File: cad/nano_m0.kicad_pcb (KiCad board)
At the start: 2 copper layers, 34.3 x 45.1 mm, 29 parts, among them J1 Conn_01x10, J2 Conn_01x10, J3 USB_B_Micro, J4 SWD, SW1 SW_SPST, SW2 SW_SPST, U1 AP2112K-3.3TRG1, U2 STM32F0706P6, Y1 16MHz

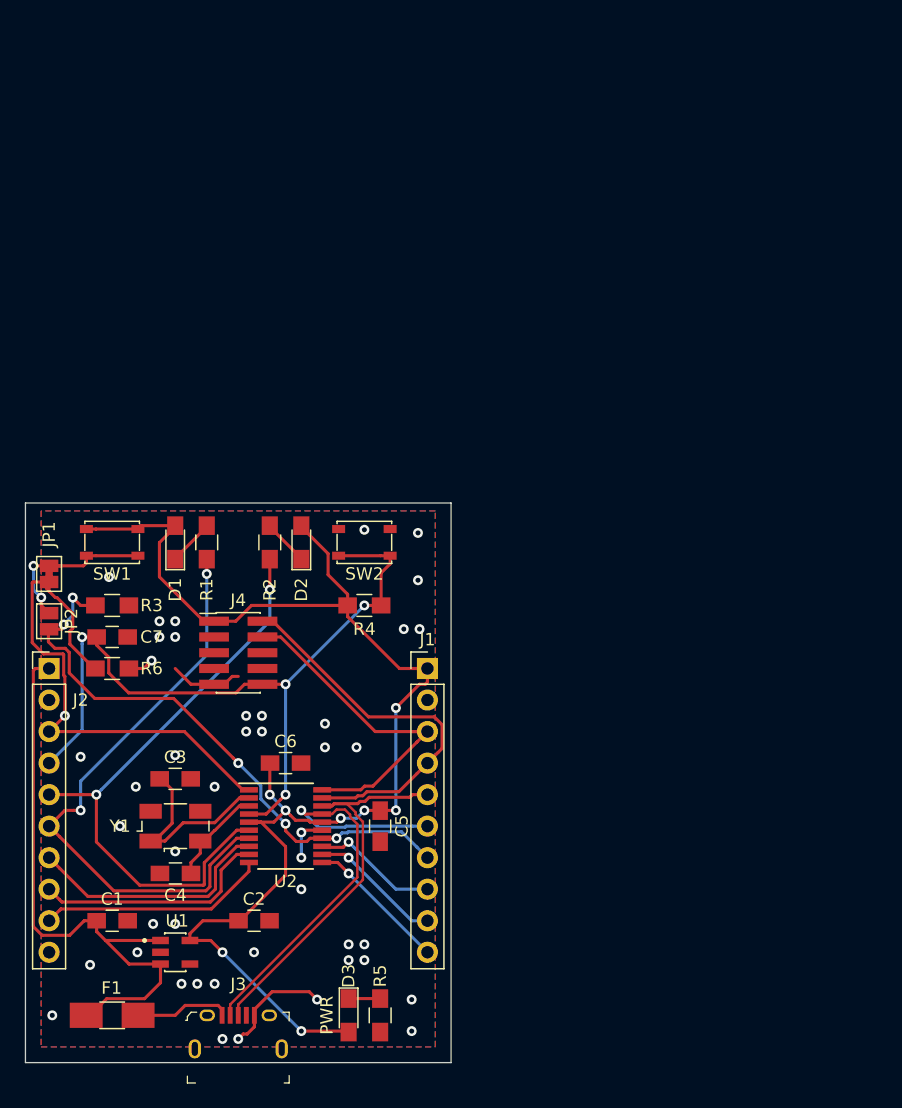
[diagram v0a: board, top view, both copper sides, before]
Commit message: board v2
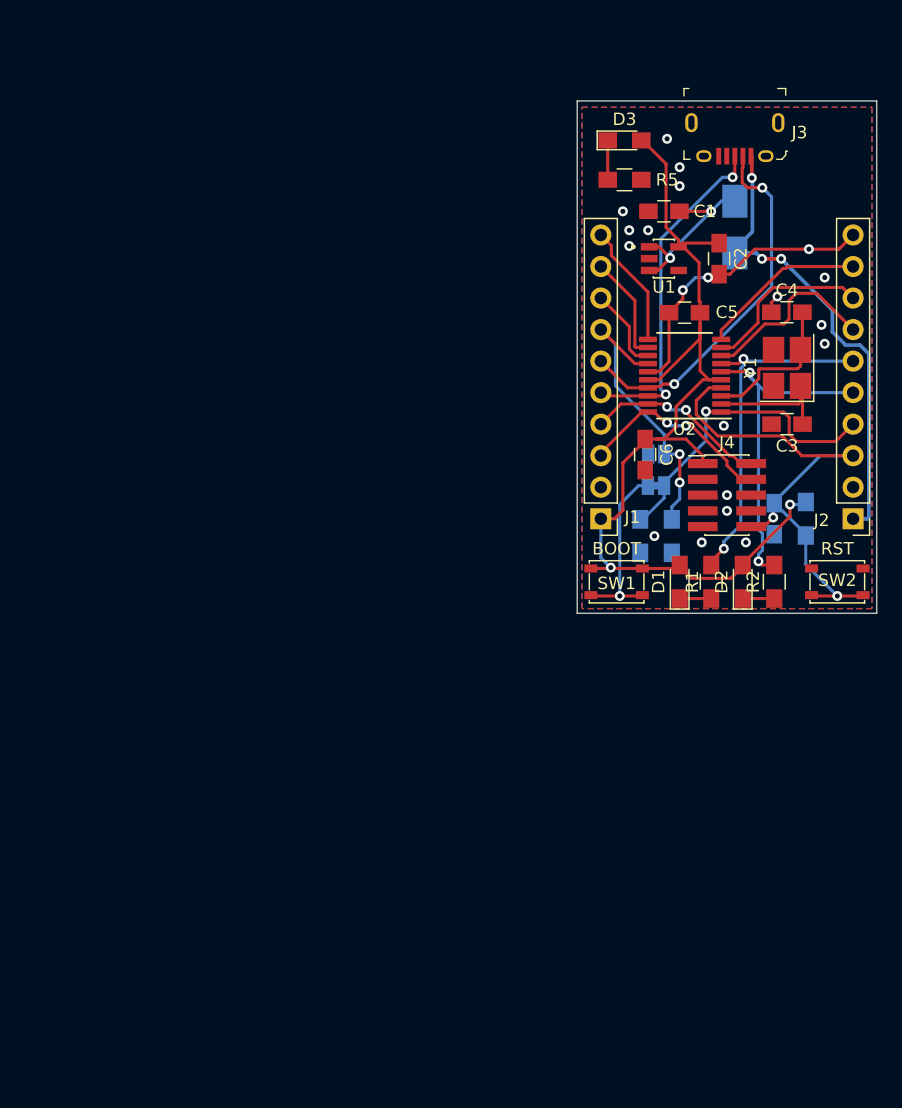
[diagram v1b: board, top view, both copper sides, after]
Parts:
- removed the REF*** at (120.0, 108.6)
- added REF***: OSHW-Symbol_6.7x6mm_SilkScreen, Symbols:OSHW-Symbol_6.7x6mm_SilkScreen, B.Cu at (143.3, 72.6)
- C3, C4: value 15pF -> 22pF
- C7, F1, JP1, JP2, R3, R4, R6: moved to B.Cu
- U1: value AP2112K-3.3TRG1 -> (none)
- Y1: value 16MHz -> Crystal; footprint Crystals:Crystal_SMD_Abracon_ABM3B-4pin_5.0x3.2mm -> Crystals:Crystal_SMD_SeikoEpson_TSX3225-4pin_3.2x2.5mm_HandSoldering
- moved F1 80.9 mm to (151.8, 78.7), turned to 270 degrees
- moved J3 79.9 mm to (151.8, 73.0), turned to 180 degrees
- moved D3 73.9 mm to (142.9, 71.8), turned to 0 degrees
- moved C1 72.4 mm to (146.1, 77.5), turned to 180 degrees
- moved R5 70.1 mm to (142.9, 74.9), turned to 0 degrees
- moved U1 68.4 mm to (146.1, 81.3)
- moved C4 66.9 mm to (156.0, 85.6)
- moved J2 65.9 mm to (161.3, 102.2), turned to 180 degrees
- moved C2 65.2 mm to (150.5, 81.3), turned to 270 degrees
- moved Y1 61.6 mm to (156.0, 90.1), turned to 90 degrees
- moved C3 57.0 mm to (156.0, 94.6), turned to 180 degrees
- moved C7 54.2 mm to (154.9, 102.2), turned to 270 degrees
- moved JP2 50.7 mm to (145.4, 97.0), turned to 0 degrees
- moved JP1 49.4 mm to (145.4, 99.6), turned to 0 degrees
- moved U2 48.5 mm to (147.7, 90.7), turned to 180 degrees
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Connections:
- C1 pad 1: +5V -> Net-(C1-Pad1)
- F1 pad 1: +5V -> Net-(C1-Pad1)
- F1 pad 2: VBUS -> +5V
- J2 pad 3: /BOOT -> /NRST
- J2 pad 4: /NRST -> /BOOT
- J3 pad 1: VBUS -> +5V
- U1 pad 1: +5V -> Net-(C1-Pad1)
- U1 pad 3: +5V -> Net-(C1-Pad1)
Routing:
- net +3V3: track 108.4 -> 81.0 mm, vias 8 -> 2
- net /PB1: track 47.4 -> 24.1 mm, vias 5 -> 2
- net /PA0: track 49.2 -> 28.4 mm
- net /PA1: track 48.5 -> 28.5 mm
- net /NRST: track 62.2 -> 42.6 mm, vias 4 -> 2
- net /BOOT: track 43.1 -> 25.2 mm
- net /PA13: track 31.1 -> 14.9 mm, vias 0 -> 2
- net Net-(C1-Pad1): track 0.00 -> 14.1 mm, vias 0 -> 2
- net /PA14: track 28.1 -> 16.5 mm, vias 0 -> 2
- net +5V: track 47.9 -> 38.1 mm, vias 0 -> 3
- net VBUS: track 7.71 -> 0.00 mm
- net /USB_N: track 35.8 -> 30.3 mm, vias 1 -> 2
- net /PA2: track 20.1 -> 14.8 mm
- net /PA3: track 19.1 -> 13.9 mm
- net /PA4: track 18.5 -> 13.5 mm
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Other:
- board size 34.3 x 45.1 mm -> 24.1 x 41.3 mm
- net class POWER added: clearance 0.25, trace_width 0.3, via_dia 0.8, via_drill 0.4
- board text added: "3.3V"
- board text added: "5V"
- board text added: "BOOT"
- board text added: "GND"
- board text added: "NANO-M0 @ZKLAPOW"
- board text added: "PA0"
- board text added: "PA1"
- board text added: "PA13"
- board text added: "PA14"
- board text added: "PA2"
- board text added: "PA3"
- board text added: "PA4"
- board text added: "PA5"
- board text added: "PA6"
- board text added: "PA7"
- board text added: "PB1"
- board text added: "RST"
- board text added: "USB_N"
- board text added: "USB_P"
- board text added: "V2"
- board text removed: "@zklapow"
- board text removed: "NANO-M0"
- board text removed: "V1"

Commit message: final v3 board
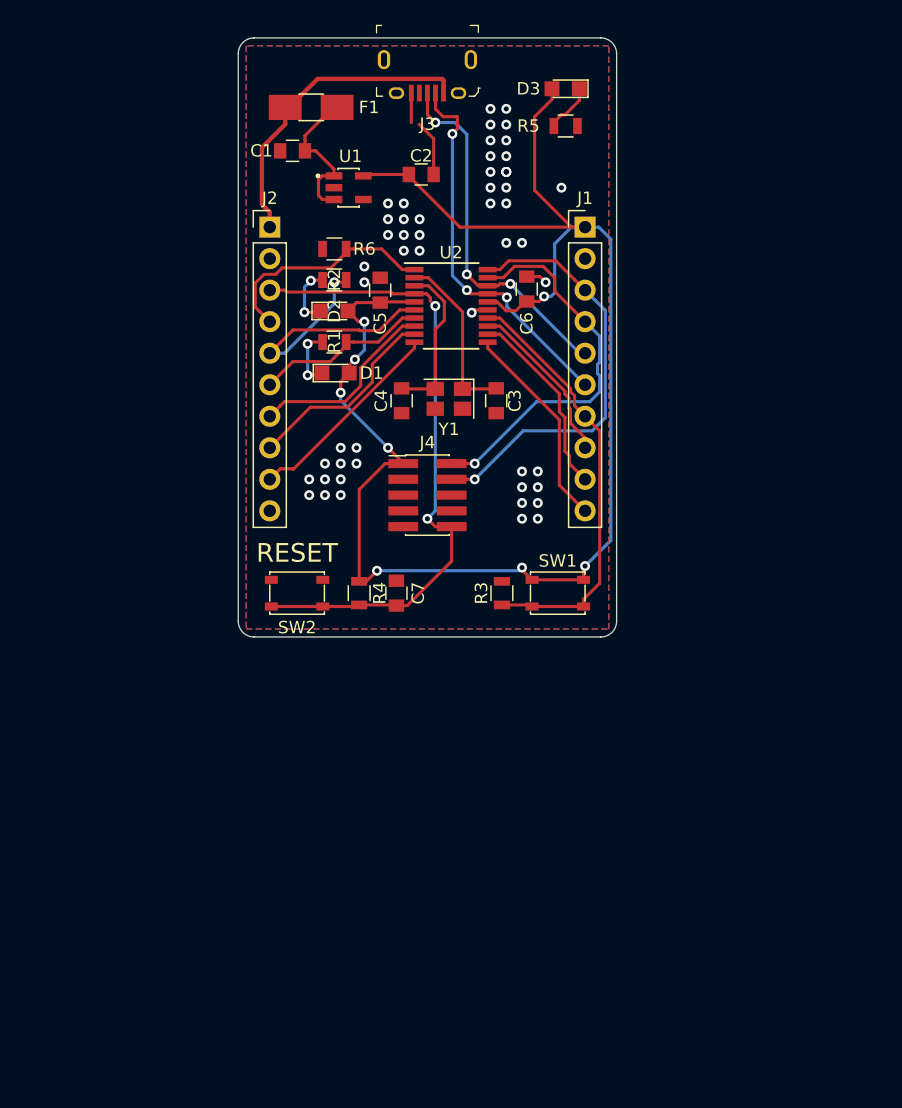
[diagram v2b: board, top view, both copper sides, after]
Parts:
- removed JP1: Jumper_NC_Small, Jumper:SolderJumper-2_P1.3mm_Bridged_Pad1.0x1.5mm
- removed JP2: Jumper_NO_Small, Jumper:SolderJumper-2_P1.3mm_Open_Pad1.0x1.5mm
- removed REF***: OSHW-Symbol_6.7x6mm_SilkScreen, Symbols:OSHW-Symbol_6.7x6mm_SilkScreen
- C1, C2, C3, C4, C5, C6: footprint Capacitors_SMD:C_0805_HandSoldering -> Capacitors_SMD:C_0805
- C7: footprint Capacitors_SMD:C_0805_HandSoldering -> Capacitors_SMD:C_0805; moved to F.Cu
- D1, D2, D3: footprint LEDs:LED_0805_HandSoldering -> LEDs:LED_0805
- F1: moved to F.Cu
- R1, R2, R5: value 80ohm -> 100; footprint Resistors_SMD:R_0805_HandSoldering -> Resistors_SMD:R_0805
- R3, R4, R6: footprint Resistors_SMD:R_0805_HandSoldering -> Resistors_SMD:R_0805; moved to F.Cu
- U1: value (none) -> AP2112K-3.3TRG1
- Y1: footprint Crystals:Crystal_SMD_SeikoEpson_TSX3225-4pin_3.2x2.5mm_HandSoldering -> Crystals:Crystal_SMD_SeikoEpson_TSX3225-4pin_3.2x2.5mm
- moved J2 52.5 mm to (114.3, 78.7), turned to 0 degrees
- moved SW2 43.5 mm to (116.5, 108.2)
- moved R2 43.0 mm to (119.5, 83.0), turned to 0 degrees
- moved D2 39.5 mm to (119.5, 85.5), turned to 0 degrees
- moved R4 36.5 mm to (121.5, 108.2)
- moved R1 36.0 mm to (119.5, 88.0), turned to 0 degrees
- moved F1 35.5 mm to (117.6, 69.1), turned to 180 degrees
- moved R6 33.8 mm to (119.5, 80.5), turned to 180 degrees
- moved D1 32.4 mm to (119.6, 90.5), turned to 0 degrees
- moved C4 31.8 mm to (124.9, 92.7), turned to 270 degrees
- moved C7 31.0 mm to (124.5, 108.2), turned to 90 degrees
- moved C1 30.3 mm to (116.1, 72.6)
- moved Y1 27.4 mm to (128.7, 92.6), turned to 180 degrees
- moved U1 26.0 mm to (120.7, 75.6)
- moved J3 25.3 mm to (127.0, 67.9)
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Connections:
- SW1 pad 2: Net-(JP1-Pad1) -> /PB1
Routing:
- net +3V3: track 81.0 -> 129.3 mm, vias 2 -> 8
- net /PA14: track 16.5 -> 34.5 mm, vias 2 -> 1
- net Net-(JP1-Pad1): track 17.5 -> 0.00 mm, vias 1 -> 0
- net /PA13: track 14.9 -> 31.3 mm, vias 2 -> 1
- net GND: track 25.3 -> 10.0 mm, vias 20 -> 52
- net /PA1: track 28.5 -> 14.1 mm, vias 2 -> 0
- net +5V: track 38.1 -> 25.5 mm, vias 3 -> 0
- net /PB1: track 24.1 -> 34.7 mm, vias 2 -> 0
- net /NRST: track 42.6 -> 52.5 mm
- net /PA7: track 6.78 -> 13.6 mm
- net /PA6: track 8.67 -> 15.5 mm
- net /PA5: track 9.99 -> 16.8 mm
- net /BOOT: track 25.2 -> 18.4 mm, vias 1 -> 0
- net /PA0: track 28.4 -> 22.7 mm, vias 2 -> 1
- net /PA4: track 13.5 -> 16.5 mm
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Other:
- board size 24.1 x 41.3 mm -> 30.5 x 48.3 mm
- net class 5v added: clearance 0.2, trace_width 0.35, via_dia 0.8, via_drill 0.4
- net class POWER removed
- board text added: "@ZKLAPOW"
- board text added: "NANO-M0"
- board text added: "RESET"
- board text added: "V3"
- board text removed: "3.3V"
- board text removed: "5V"
- board text removed: "BOOT"
- board text removed: "GND"
- board text removed: "NANO-M0 @ZKLAPOW"
- board text removed: "PA0"
- board text removed: "PA1"
- board text removed: "PA13"
- board text removed: "PA14"
- board text removed: "PA2"
- board text removed: "PA3"
- board text removed: "PA4"
- board text removed: "PA5"
- board text removed: "PA6"
- board text removed: "PA7"
- board text removed: "PB1"
- board text removed: "RST"
- board text removed: "USB_N"
- board text removed: "USB_P"
- board text removed: "V2"
